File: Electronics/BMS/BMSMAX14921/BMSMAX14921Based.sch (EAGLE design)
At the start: 66 parts, among them IC1 MAX14921, J1 CONNECTOR_9PIN, J4 CONNECTOR_9PIN, J5 CONNECTOR_8PIN, J6 CONNECTOR_9PIN

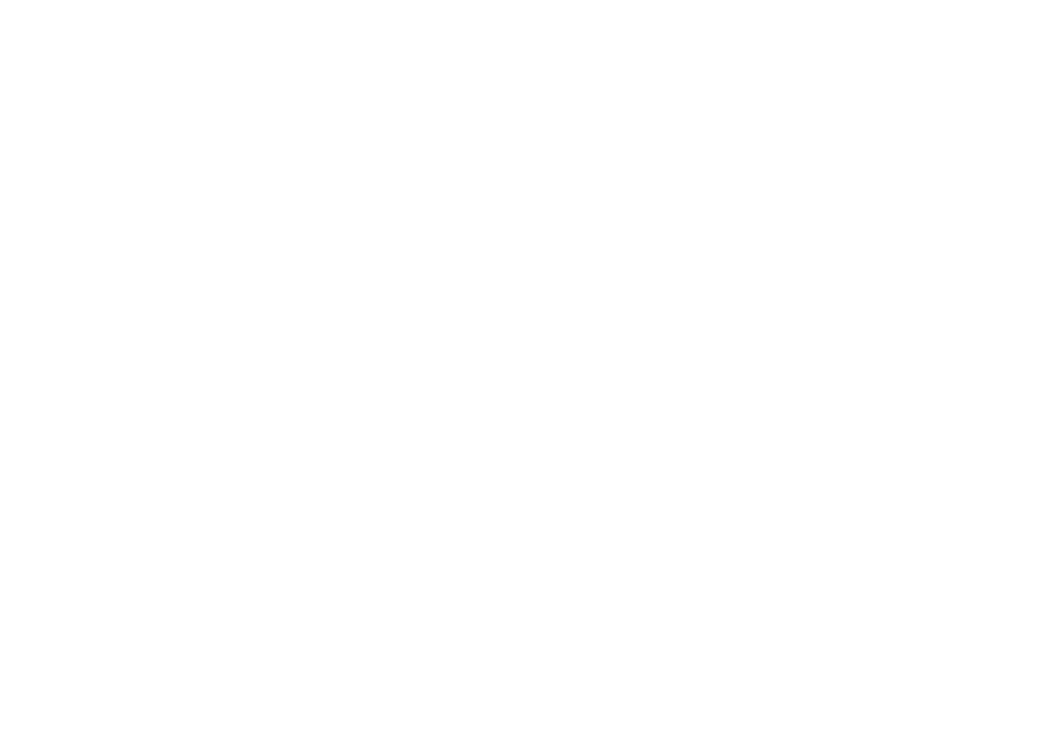
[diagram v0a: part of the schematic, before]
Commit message: dank work bean
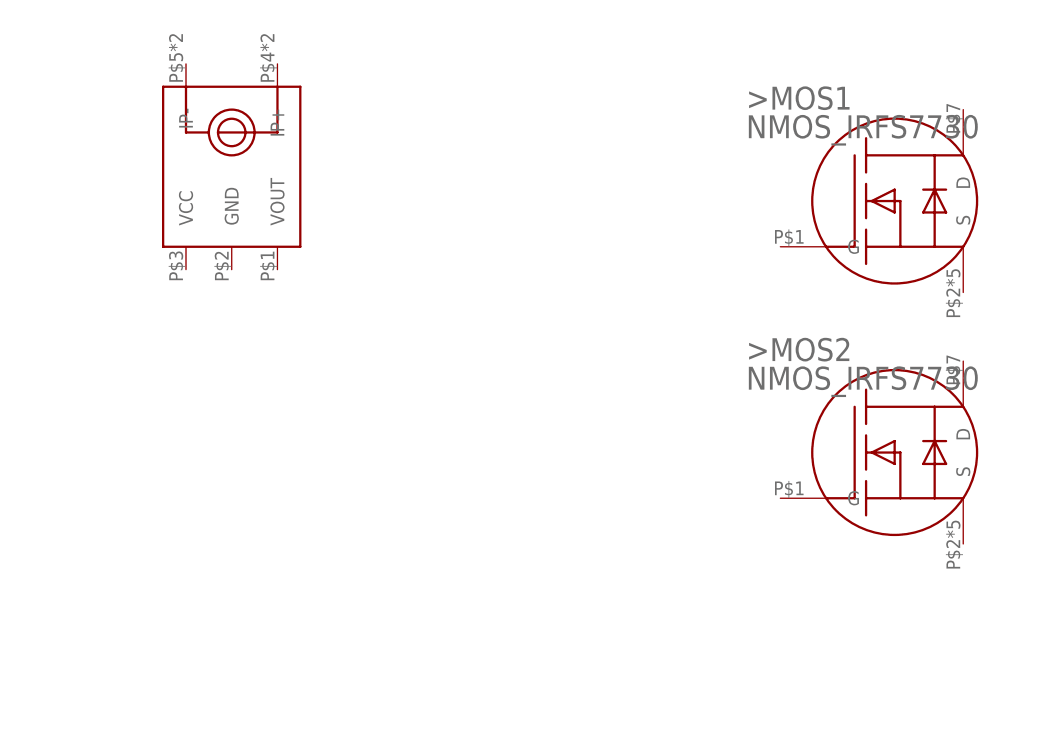
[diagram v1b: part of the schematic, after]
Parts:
- added >MOS1, >MOS2: NMOS_IRFS7730, MarkIIEaglelbr:NMOS_IRFS7730
- added U$1: ACS758XCB, MarkIIEaglelbr:ACS758XCB
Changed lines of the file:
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@@
 <part name="J5" library="lolomolo" deviceset="CONNECTOR_8PIN" device=""/>
 <part name="J6" library="lolomolo" deviceset="CONNECTOR_9PIN" device=""/>
+<part name="U$1" library="MarkIIEaglelbr" deviceset="ACS758XCB" device=""/>
+<part name="&gt;MOS1" library="MarkIIEaglelbr" deviceset="NMOS_IRFS7730" device=""/>
+<part name="&gt;MOS2" library="MarkIIEaglelbr" deviceset="NMOS_IRFS7730" device=""/>
 </parts>
 <sheets>
@@
 <instance part="J5" gate="G$1" x="-177.8" y="33.02" rot="R180"/>
 <instance part="J6" gate="G$1" x="-175.26" y="55.88" rot="MR0"/>
+<instance part="U$1" gate="G$1" x="223.52" y="111.76"/>
+<instance part="&gt;MOS1" gate="G$1" x="297.18" y="109.22"/>
+<instance part="&gt;MOS2" gate="G$1" x="297.18" y="81.28"/>
 </instances>
 <busses>
